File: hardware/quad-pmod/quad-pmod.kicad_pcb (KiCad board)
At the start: 2 copper layers, 52.1 x 27.9 mm, 9 parts, among them J1 PMOD, J2 PMOD, J3 S7 Mini, J4 S7 Mini, J5 PWR, J6 PWR, J7 PMOD, J8 PMOD

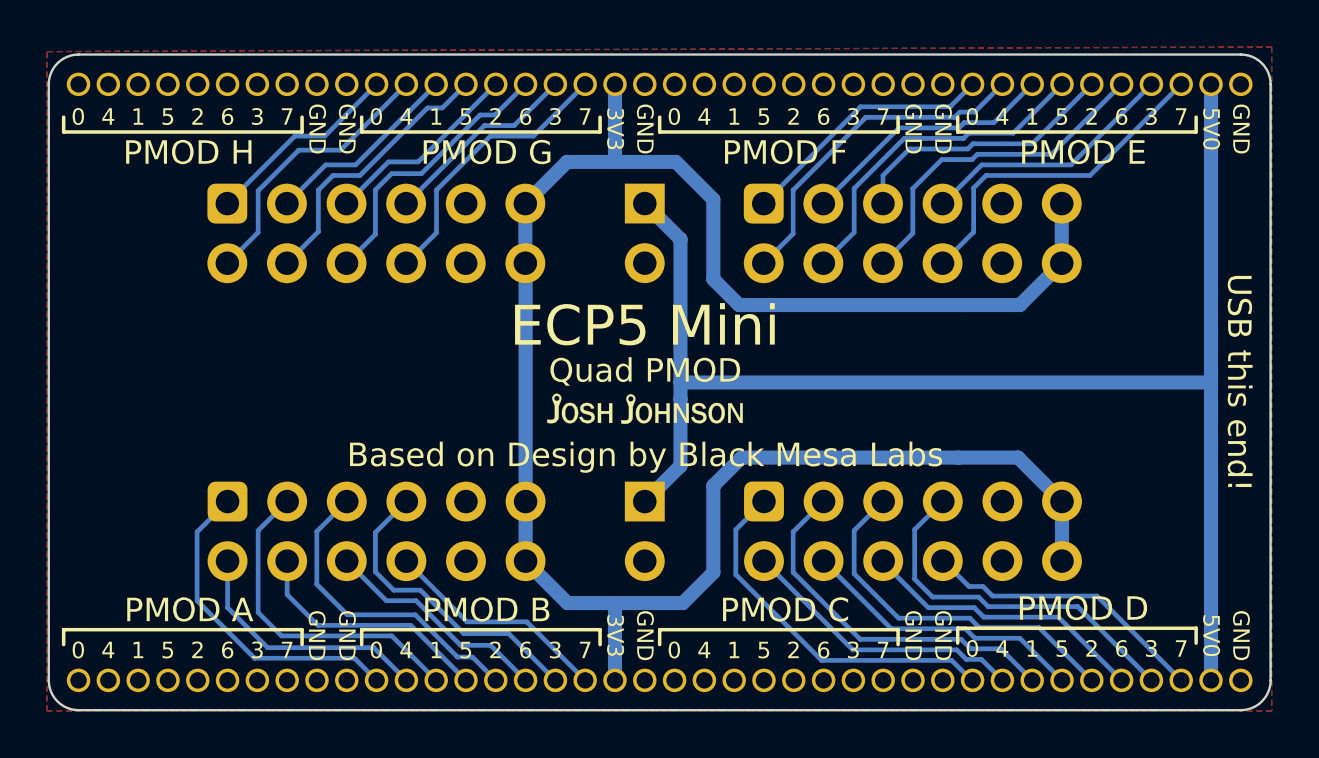
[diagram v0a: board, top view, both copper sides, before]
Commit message: clean up routing
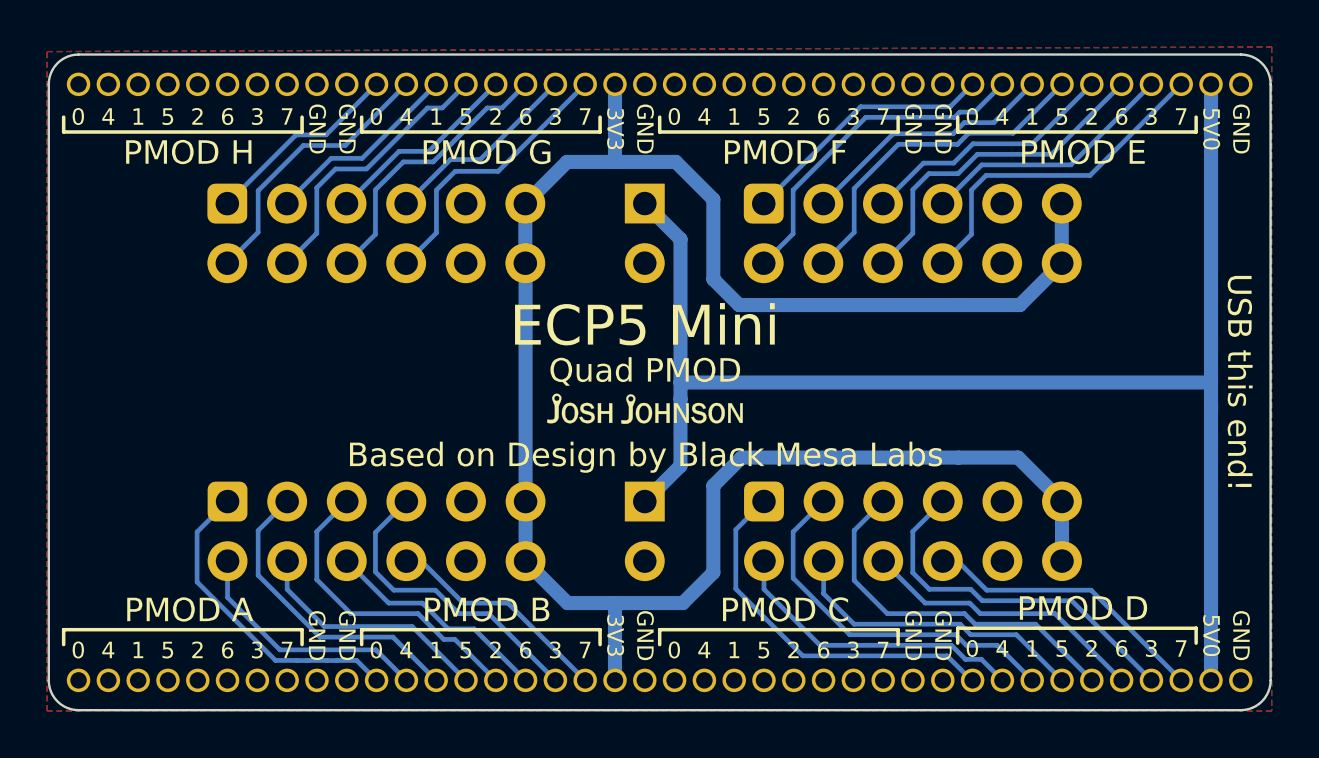
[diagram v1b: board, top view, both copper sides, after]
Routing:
- net /PORT_B1: track 14.0 -> 13.1 mm
- net /PORT_D5: track 12.3 -> 13.1 mm
- net /PORT_E2: track 11.7 -> 11.0 mm
- net /PORT_D4: track 12.3 -> 13.0 mm
